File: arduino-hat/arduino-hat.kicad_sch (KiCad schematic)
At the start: 20 parts, among them Q1 MMBT2222A, Q2 MMBT2222A, Q3 MMBT2222A, Q4 MMBT2222A

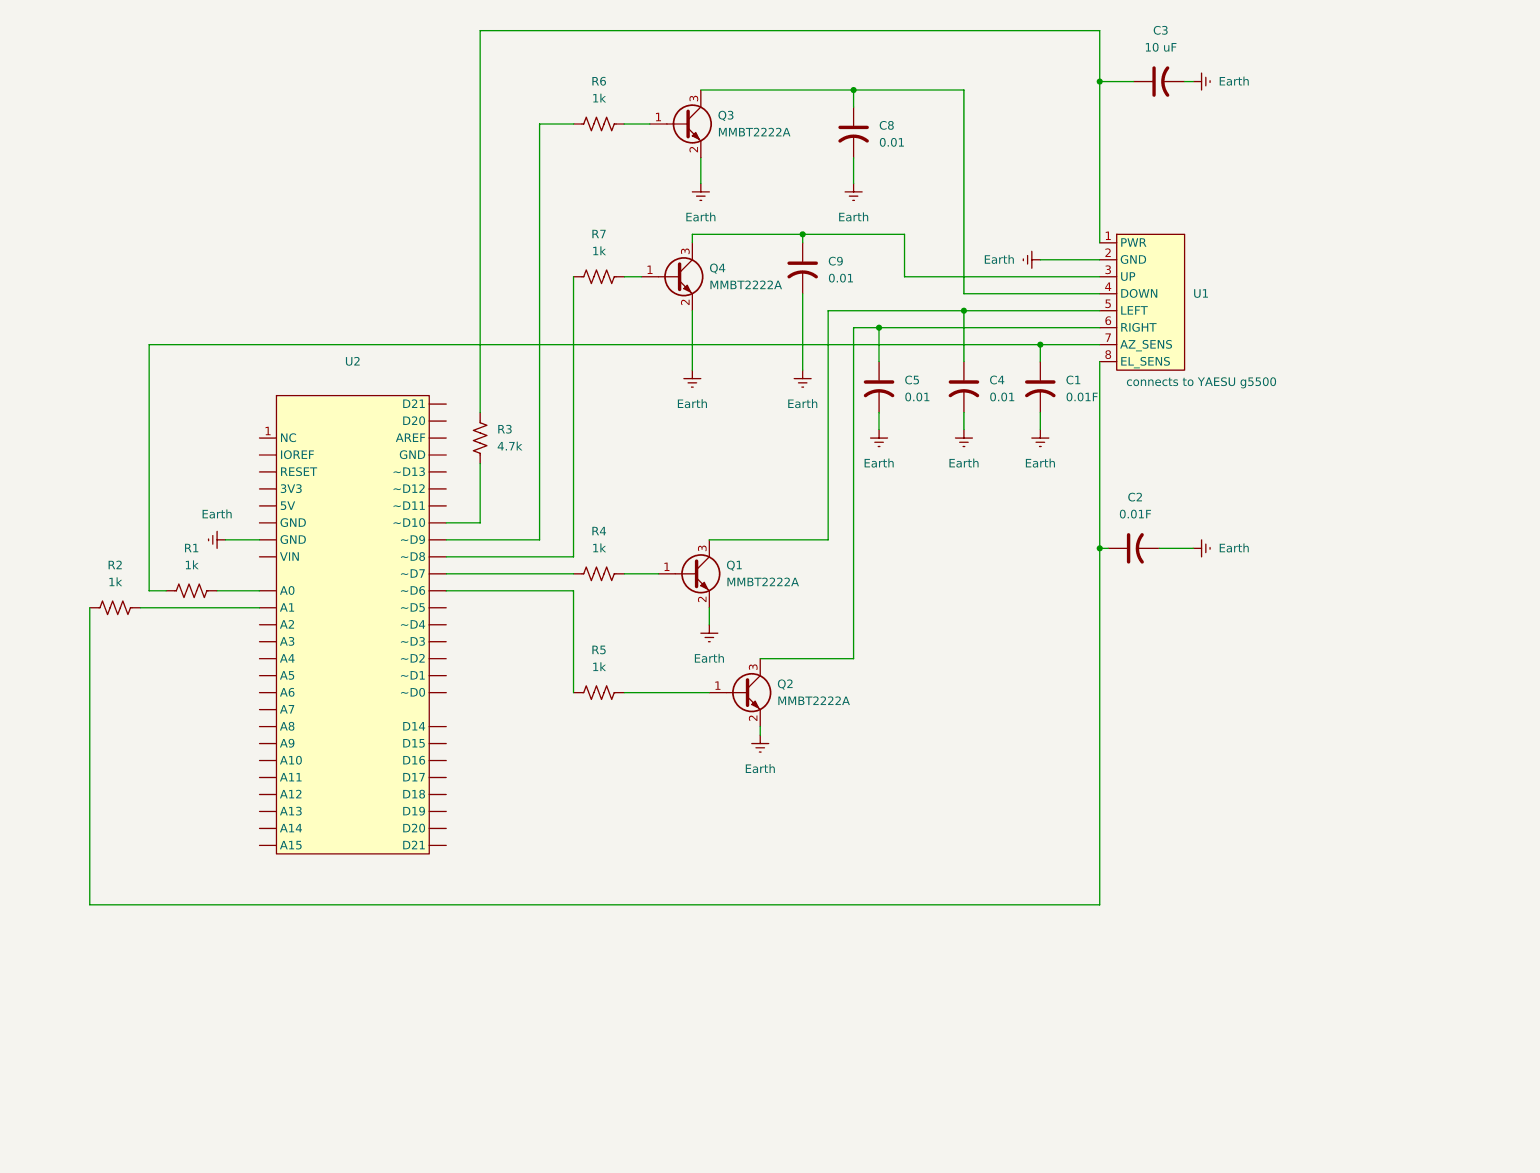
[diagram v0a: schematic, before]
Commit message: finished schematic?
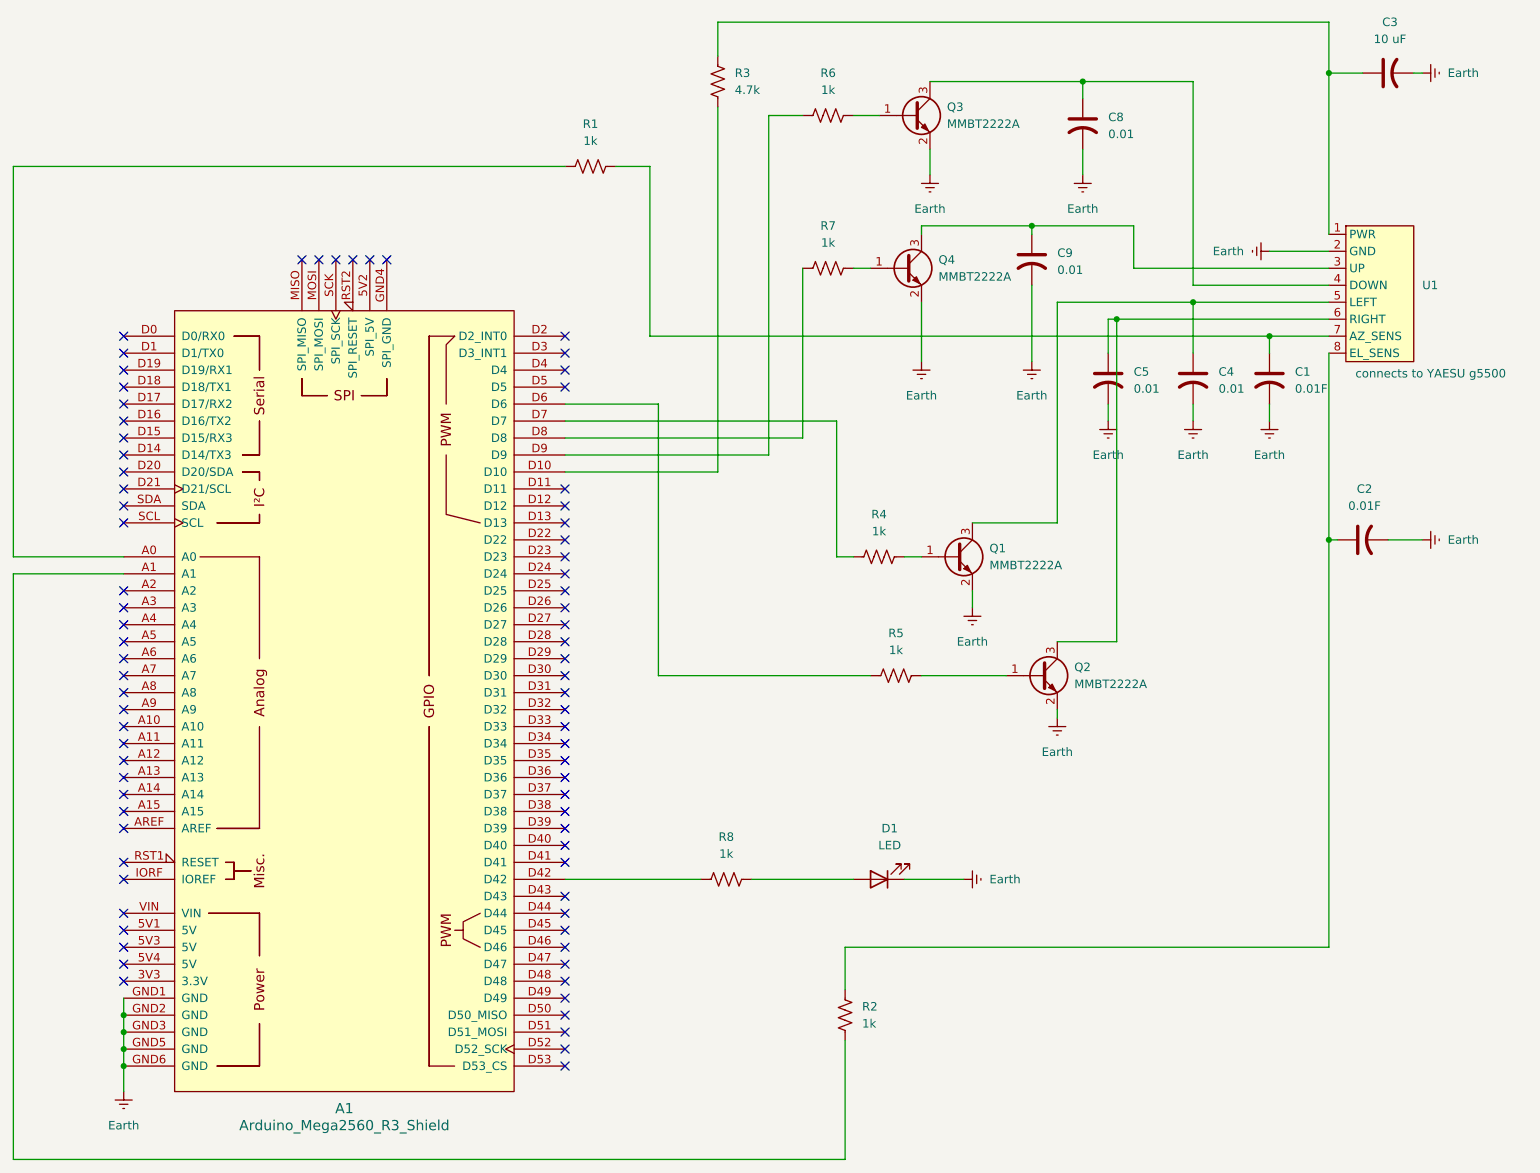
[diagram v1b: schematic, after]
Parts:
- removed U2: ~, symbol connectors:arduinoMEGA_hat_pins
- added A1: Arduino_Mega2560_R3_Shield, PCM_arduino-library:Arduino_Mega2560_R3_Shield, symbol PCM_arduino-library:Arduino_Mega2560_R3_Shield
- added D1: LED, LED_SMD:LED_1210_3225Metric_Pad1.42x2.65mm_HandSolder, symbol Device:LED
- added R8: 1k, Resistor_SMD:R_1210_3225Metric_Pad1.30x2.65mm_HandSolder, symbol Device:R_US
- C1, C2, C3, C4, C5, C8, C9: footprint (none) -> Capacitor_SMD:C_1210_3225Metric_Pad1.33x2.70mm_HandSolder
- R1, R2, R3, R4, R5, R6, R7: footprint (none) -> Resistor_SMD:R_1210_3225Metric_Pad1.30x2.65mm_HandSolder
- U1: footprint (none) -> Connector_PinHeader_2.54mm:PinHeader_1x08_P2.54mm_Vertical
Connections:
- net Earth: now also A1.GND1 (GND), A1.GND2 (GND), A1.GND3 (GND), A1.GND5 (GND), A1.GND6 (GND), D1.1 (K)
- net at C1.1, U1.7 (AZ_SENS): now also R1.2; no longer R1.1
- net at R2.2: now also A1.A1
- net at R5.1: now also A1.D6
- net at R4.1: now also A1.D7
- net at R6.1: now also A1.D9
- net at R3.2: now also A1.D10
- net at R7.1: now also A1.D8
- new net: A1.A0, R1.1
- new net: A1.D42, R8.2
- new net: D1.2 (A), R8.1
- no-connect marks 0 -> 78
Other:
- moved on the sheet: C1, C2, C3, C4, C5, C8, C9, Q1, Q2, Q3, Q4, R1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
